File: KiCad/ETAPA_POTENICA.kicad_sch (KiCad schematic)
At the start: 14 parts, among them U3 VNH5019A-E, U5 VNH5019A-E

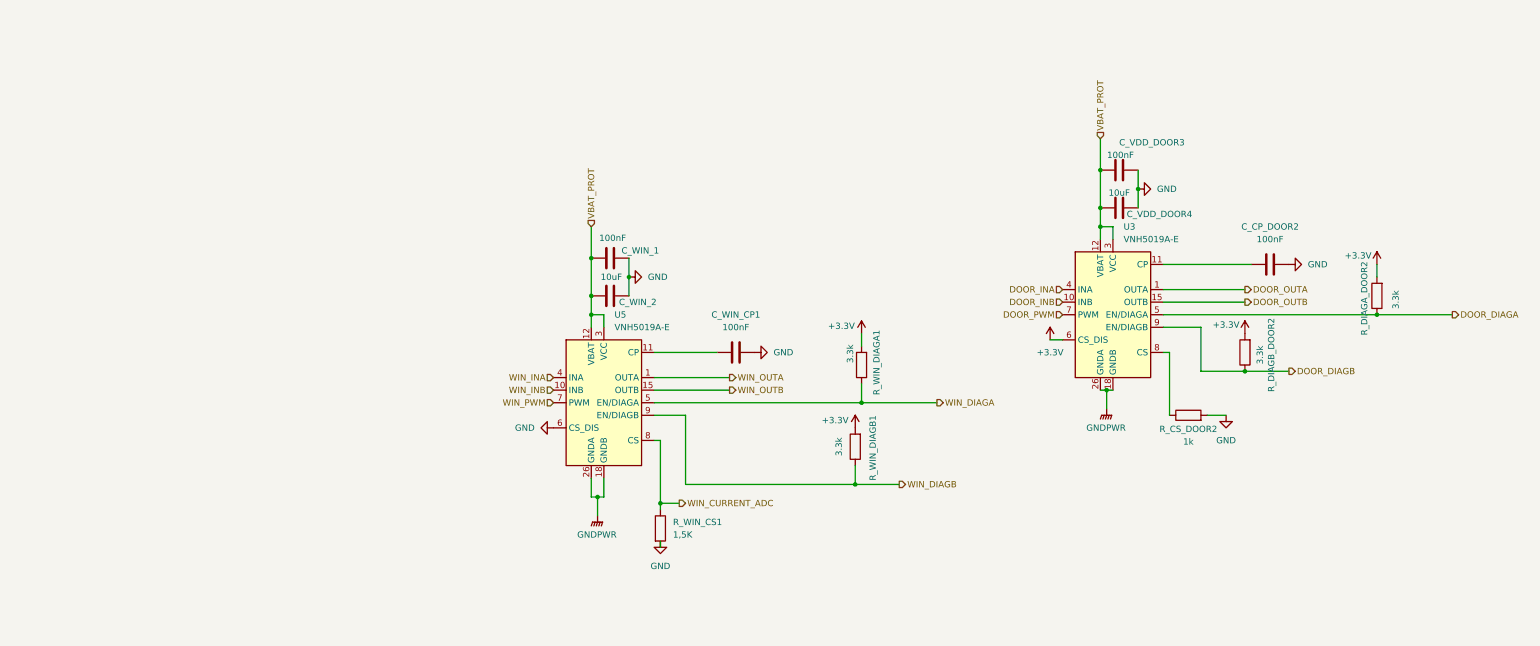
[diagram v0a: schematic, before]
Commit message: Versió final Esquematic
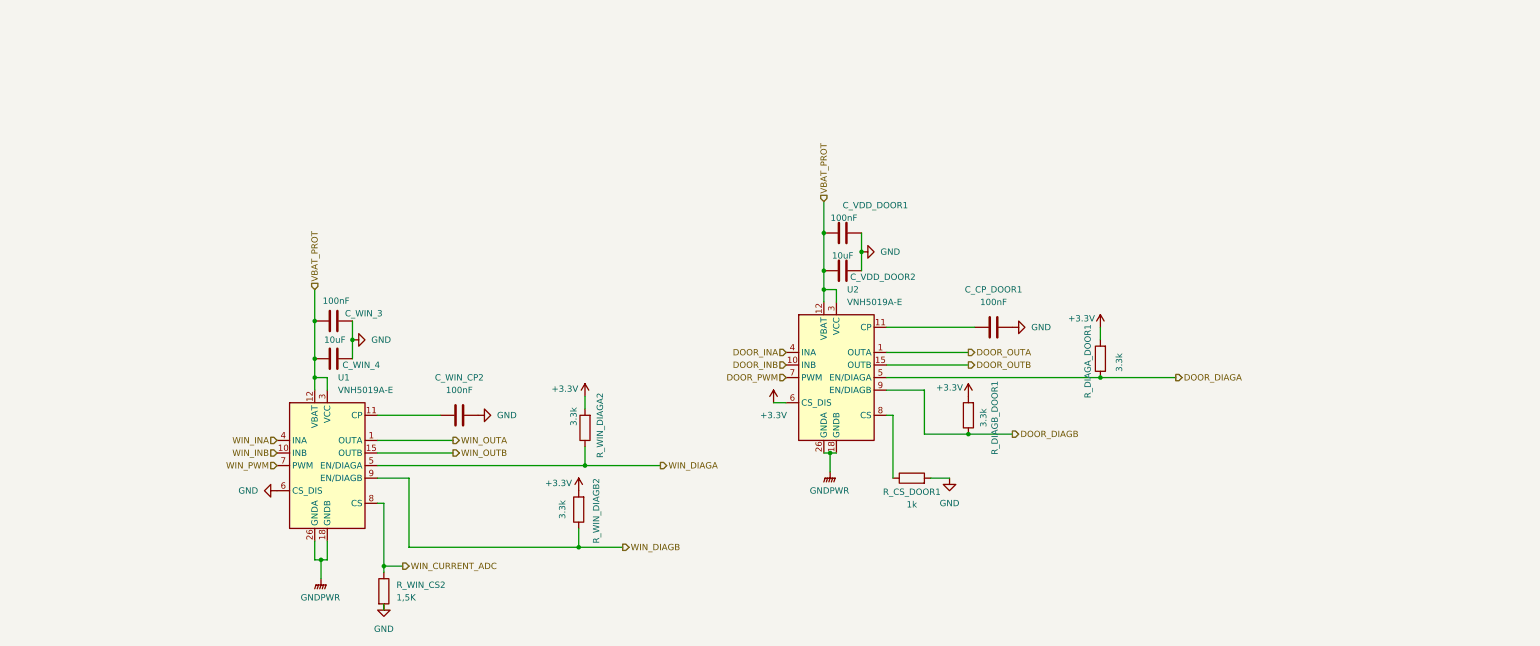
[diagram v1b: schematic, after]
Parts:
- removed C_CP_DOOR2, C_VDD_DOOR3, C_WIN_1, C_WIN_CP1: 100nF, Capacitor_SMD:C_0805_2012Metric, symbol Device:C
- removed C_VDD_DOOR4: 10uF, Capacitor_SMD:CP_Elec_8x10, symbol Device:C
- removed C_WIN_2: 10uF, Capacitor_SMD:C_1206_3216Metric, symbol Device:C
- removed R_CS_DOOR2: 1k, Resistor_SMD:R_0805_2012Metric, symbol Device:R
- removed R_DIAGA_DOOR2, R_DIAGB_DOOR2, R_WIN_DIAGA1, R_WIN_DIAGB1: 3.3k, Resistor_SMD:R_0805_2012Metric, symbol Device:R
- removed R_WIN_CS1: 1,5K, Resistor_SMD:R_0805_2012Metric, symbol Device:R
- removed U3, U5: VNH5019A-E, Package_SO:ST_MultiPowerSO-30, symbol Driver_Motor:VNH5019A-E
- added C_CP_DOOR1, C_VDD_DOOR1, C_WIN_3, C_WIN_CP2: 100nF, Capacitor_SMD:C_0805_2012Metric, symbol Device:C
- added C_VDD_DOOR2: 10uF, Capacitor_SMD:CP_Elec_8x10, symbol Device:C
- added C_WIN_4: 10uF, Capacitor_SMD:C_1206_3216Metric, symbol Device:C
- added R_CS_DOOR1: 1k, Resistor_SMD:R_0805_2012Metric, symbol Device:R
- added R_DIAGA_DOOR1, R_DIAGB_DOOR1, R_WIN_DIAGA2, R_WIN_DIAGB2: 3.3k, Resistor_SMD:R_0805_2012Metric, symbol Device:R
- added R_WIN_CS2: 1,5K, Resistor_SMD:R_0805_2012Metric, symbol Device:R
- added U1, U2: VNH5019A-E, Package_SO:ST_MultiPowerSO-30, symbol Driver_Motor:VNH5019A-E
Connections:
- net +3.3V: now also R_DIAGA_DOOR1.2, R_DIAGB_DOOR1.2, R_WIN_DIAGA2.2, R_WIN_DIAGB2.2, U2.6 (CS_DIS)
- net DOOR_DIAGA: now also R_DIAGA_DOOR1.1, U2.5 (EN/DIAGA)
- net DOOR_DIAGB: now also R_DIAGB_DOOR1.1, U2.9 (EN/DIAGB)
- net DOOR_INA: now also U2.4 (INA)
- net DOOR_INB: now also U2.10 (INB)
- net DOOR_OUTA: now also U2.1 (OUTA), U2.25 (OUTA), U2.30 (OUTA), U2.33 (OUTA)
- net DOOR_OUTB: now also U2.15 (OUTB), U2.16 (OUTB), U2.21 (OUTB), U2.32 (OUTB)
- net DOOR_PWM: now also U2.7 (PWM)
- net GND: now also C_CP_DOOR1.1, C_VDD_DOOR1.2, C_VDD_DOOR2.2, C_WIN_3.2, C_WIN_4.2, C_WIN_CP2.1, R_CS_DOOR1.2, R_WIN_CS2.2, U1.6 (CS_DIS)
- net GNDPWR: now also U1.18 (GNDB), U1.19 (GNDB), U1.20 (GNDB), U1.26 (GNDA), U1.27 (GNDA), U1.28 (GNDA), U2.18 (GNDB), U2.19 (GNDB), U2.20 (GNDB), U2.26 (GNDA), U2.27 (GNDA), U2.28 (GNDA)
- net VBAT_PROT: now also C_VDD_DOOR1.1, C_VDD_DOOR2.1, C_WIN_3.1, C_WIN_4.1, U1.12 (VBAT), U1.13 (VCC), U1.23 (VCC), U1.3 (VCC), U1.31 (VCC), U2.12 (VBAT), U2.13 (VCC), U2.23 (VCC), U2.3 (VCC), U2.31 (VCC)
- net WIN_CURRENT_ADC: now also R_WIN_CS2.1, U1.8 (CS)
- net WIN_DIAGA: now also R_WIN_DIAGA2.1, U1.5 (EN/DIAGA)
- net WIN_DIAGB: now also R_WIN_DIAGB2.1, U1.9 (EN/DIAGB)
- net WIN_INA: now also U1.4 (INA)
- net WIN_INB: now also U1.10 (INB)
- net WIN_OUTA: now also U1.1 (OUTA), U1.25 (OUTA), U1.30 (OUTA), U1.33 (OUTA)
- net WIN_OUTB: now also U1.15 (OUTB), U1.16 (OUTB), U1.21 (OUTB), U1.32 (OUTB)
- net WIN_PWM: now also U1.7 (PWM)
- new net: C_WIN_CP2.2, U1.11 (CP)
- new net: R_CS_DOOR1.1, U2.8 (CS)
- new net: C_CP_DOOR1.2, U2.11 (CP)

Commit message: Versió final de l'esquematic
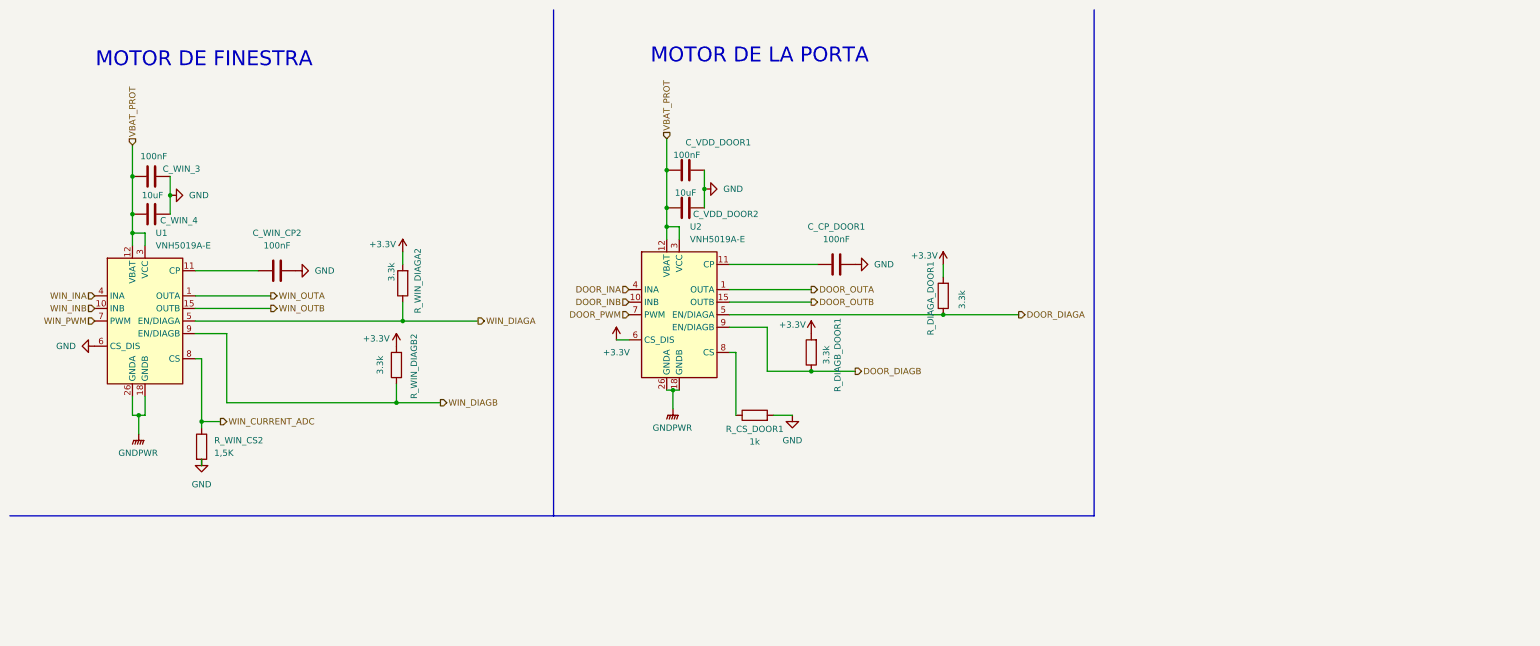
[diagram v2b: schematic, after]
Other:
- note added: "MOTOR DE FINESTRA"
- note added: "MOTOR DE LA PORTA"
- moved on the sheet: C_CP_DOOR1, C_VDD_DOOR1, C_VDD_DOOR2, C_WIN_3, C_WIN_4, C_WIN_CP2, R_CS_DOOR1, R_DIAGA_DOOR1, R_DIAGB_DOOR1, R_WIN_CS2, R_WIN_DIAGA2, R_WIN_DIAGB2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
